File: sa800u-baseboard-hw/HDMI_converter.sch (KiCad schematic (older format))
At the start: 17 parts, among them U4 LT9611, Y2 ECS-1618-250-BN-TR

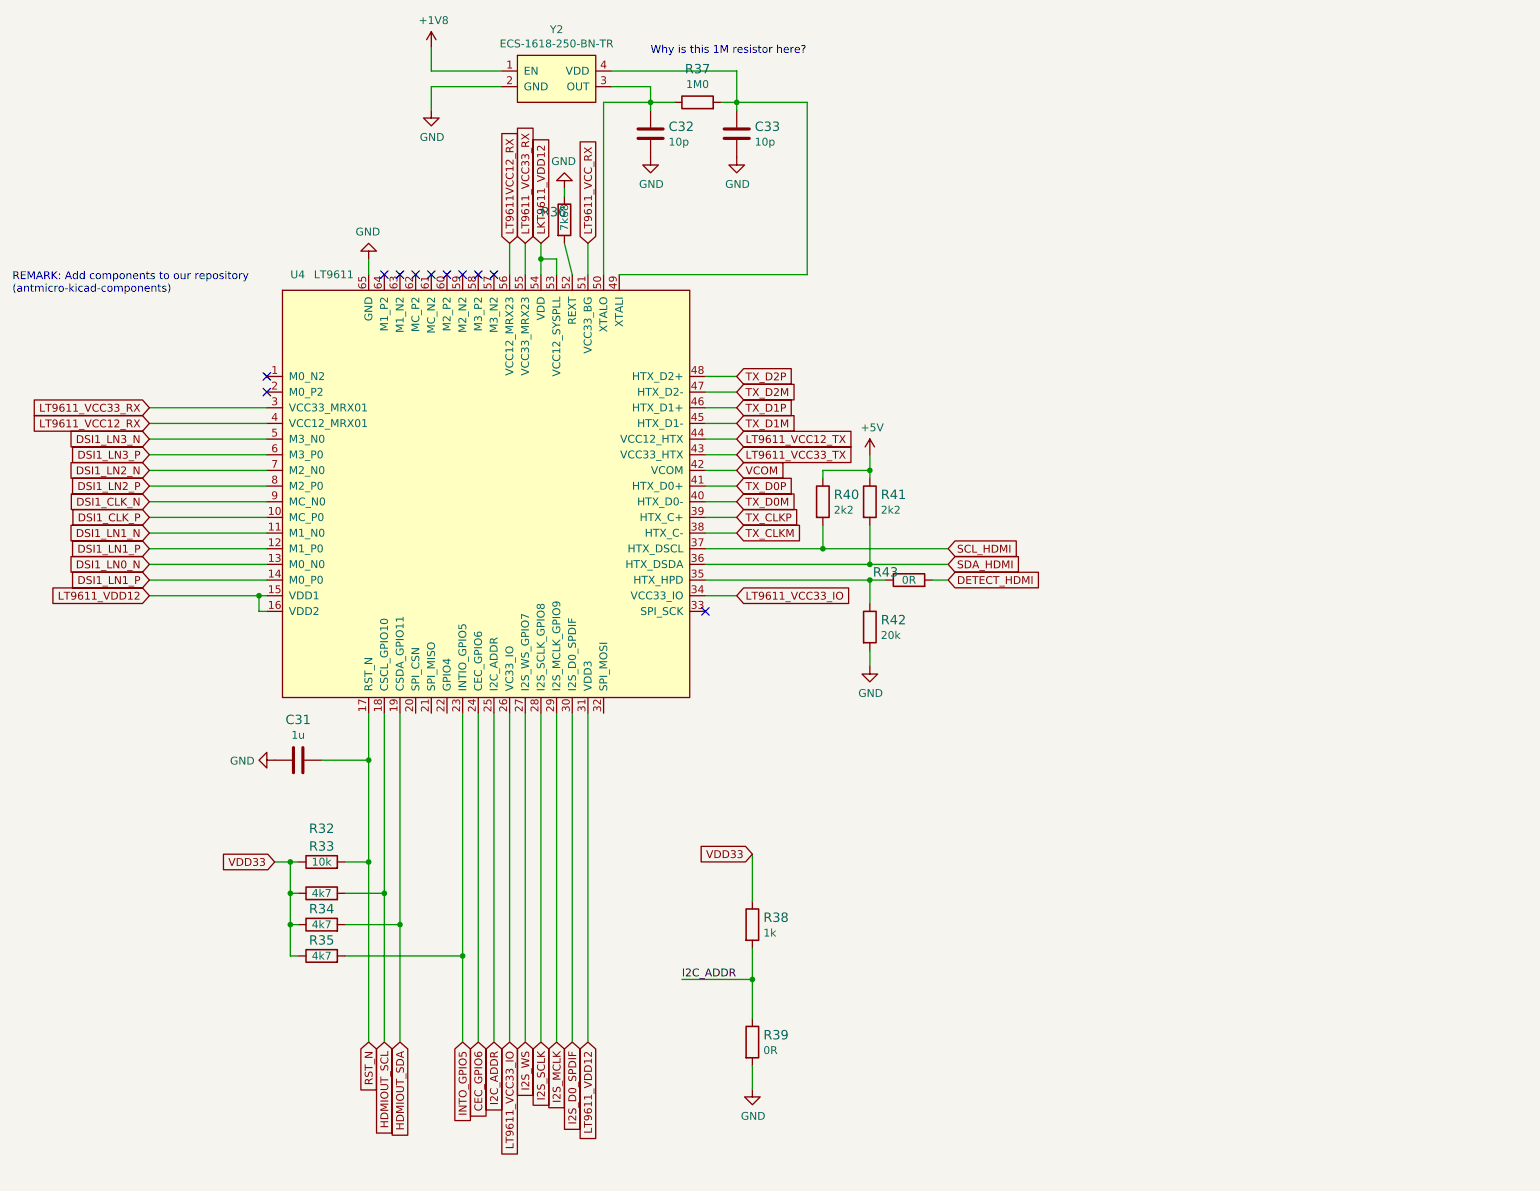
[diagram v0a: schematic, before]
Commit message: introducing minor genreal improvements
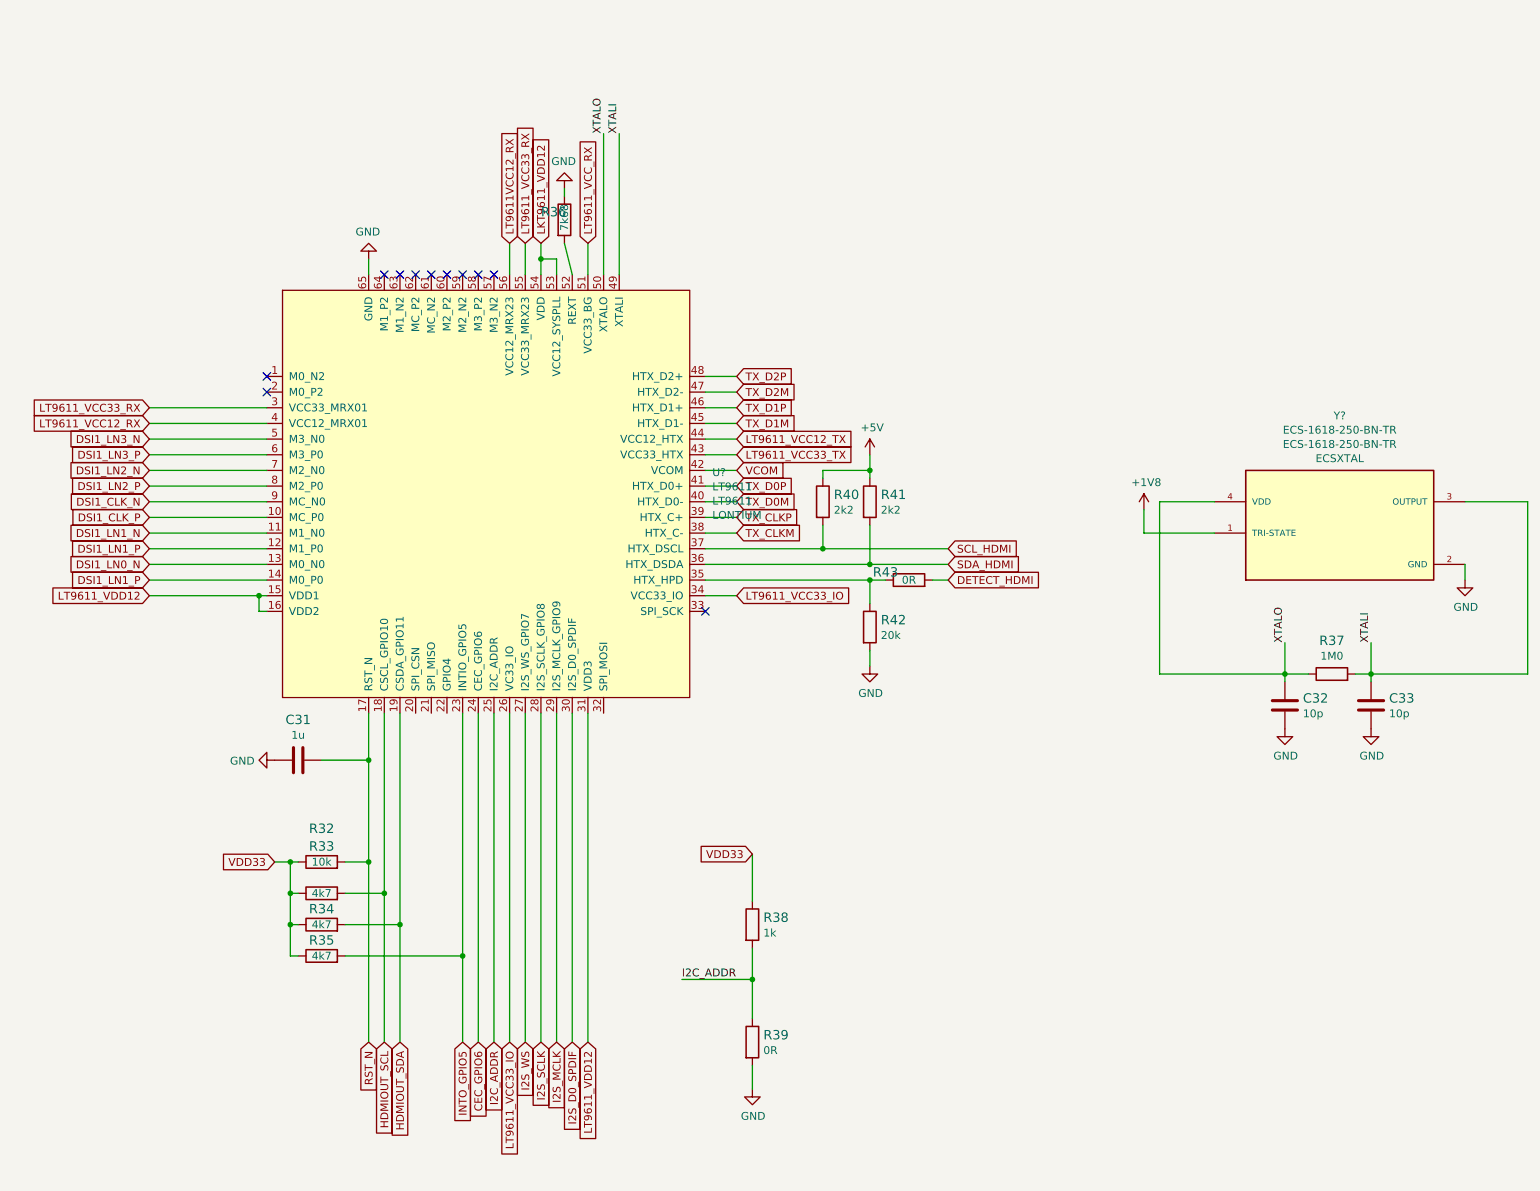
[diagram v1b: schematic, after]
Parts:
- removed U4: LT9611, symbol HDMI:LT9611
- removed Y2: ECS-1618-250-BN-TR, symbol Oscillators:ECS-1618-250-BN-TR
- added U?: LT9611, antmicro-footprints:LT9611, symbol antmicroInterfaceControllers:LT9611
- added Y?: ECS-1618-250-BN-TR, antmicro-footprints:OSC_ECS-1618-250-BN-TR, symbol antmicroOscillators:ECS-1618-250-BN-TR
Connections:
- net +1V8: now also Y?.1 (TRI-STATE)
- net CEC_GPIO6: now also U?.24 (CEC_GPIO6)
- net DSI1_CLK_N: now also U?.9 (MC_N0)
- net DSI1_CLK_P: now also U?.10 (MC_P0)
- net DSI1_LN0_N: now also U?.13 (M0_N0)
- net DSI1_LN1_N: now also U?.11 (M1_N0)
- net DSI1_LN1_P: now also U?.12 (M1_P0), U?.14 (M0_P0)
- net DSI1_LN2_N: now also U?.7 (M2_N0)
- net DSI1_LN2_P: now also U?.8 (M2_P0)
- net DSI1_LN3_N: now also U?.5 (M3_N0)
- net DSI1_LN3_P: now also U?.6 (M3_P0)
- net GND: now also U?.65 (GND), Y?.2 (GND)
- net HDMIOUT_SCL: now also U?.18 (CSCL_GPIO10)
- net HDMIOUT_SDA: now also U?.19 (CSDA_GPIO11)
- net I2C_ADDR: now also U?.25 (I2C_ADDR)
- net I2S_D0_SPDIF: now also U?.30 (I2S_D0_SPDIF)
- net I2S_MCLK: now also U?.29 (I2S_MCLK_GPIO9)
- net I2S_SCLK: now also U?.28 (I2S_SCLK_GPIO8)
- net I2S_WS: now also U?.27 (I2S_WS_GPIO7)
- net INTO_GPIO5: now also U?.23 (INTIO_GPIO5)
- net LKT9611_VDD12: now also U?.53 (VCC12_SYSPLL), U?.54 (VDD)
- net LT9611VCC12_RX: now also U?.56 (VCC12_MRX23)
- net LT9611_VCC12_RX: now also U?.4 (VCC12_MRX01)
- net LT9611_VCC12_TX: now also U?.44 (VCC12_HTX)
- net LT9611_VCC33_IO: now also U?.26 (VC33_IO), U?.34 (VCC33_IO)
- net LT9611_VCC33_RX: now also U?.3 (VCC33_MRX01), U?.55 (VCC33_MRX23)
- net LT9611_VCC33_TX: now also U?.43 (VCC33_HTX)
- net LT9611_VCC_RX: now also U?.51 (VCC33_BG)
- net LT9611_VDD12: now also U?.15 (VDD1), U?.16 (VDD2), U?.31 (VDD3)
- net RST_N: now also U?.17 (RST_N)
- net SCL_HDMI: now also U?.37 (HTX_DSCL)
- net SDA_HDMI: now also U?.36 (HTX_DSDA)
- net TX_CLKM: now also U?.38 (HTX_C-)
- net TX_CLKP: now also U?.39 (HTX_C+)
- net TX_D0M: now also U?.40 (HTX_D0-)
- net TX_D0P: now also U?.41 (HTX_D0+)
- net TX_D1M: now also U?.45 (HTX_D1-)
- net TX_D1P: now also U?.46 (HTX_D1+)
- net TX_D2M: now also U?.47 (HTX_D2-)
- net TX_D2P: now also U?.48 (HTX_D2+)
- net VCOM: now also U?.42 (VCOM)
- net at R42.1, R43.1: now also U?.35 (HTX_HPD)
- net XTALI: now reaches C33.1, R37.2
- net XTALI: now also U?.49 (XTALI), Y?.3 (OUTPUT)
- net XTALO: now reaches C32.1, R37.1
- net XTALO: now also U?.50 (XTALO), Y?.4 (VDD)
- net at R36.2: now also U?.52 (REXT)
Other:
- note removed: "REMARK: Add components to our repository \n(antmicro-kicad-components)"
- note removed: "Why is this 1M resistor here? \n"
- moved on the sheet: C32, C33, R37
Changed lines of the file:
@@
 Comment4 ""
 $EndDescr
-$Comp
-L HDMI:LT9611 U4
-U 1 1 61A0479A
-P 2250 2250
-F 0 "U4" H 2300 2350 50  0000 L CNN
-F 1 "LT9611" H 2450 2350 50  0000 L CNN
-F 2 "" H 1500 1950 50  0001 C CNN
-F 3 "" H 1500 1950 50  0001 C CNN
-	1    2250 2250
-	1    0    0    -1
-$EndComp
 Wire Wire Line
 	1400 3000 2150 3000
@@
 L power:GND #PWR?
 U 1 1 61A80E9F
-P 3200 1100
+P 9800 4100
 AR Path="/618E716E/61A80E9F" Ref="#PWR?"  Part="1"
 AR Path="/6197686D/61A80E9F" Ref="#PWR0115"  Part="1"
-F 0 "#PWR0115" H 3200 850 50  0001 C CNN
-F 1 "GND" H 3205 927 50  0000 C CNN
-F 2 "" H 3200 1100 50  0001 C CNN
-F 3 "" H 3200 1100 50  0001 C CNN
-	1    3200 1100
-	1    0    0    -1
-$EndComp
-Wire Wire Line
-	3200 950  3200 1100
-Wire Wire Line
-	3650 950  3200 950
+F 0 "#PWR0115" H 9800 3850 50  0001 C CNN
+F 1 "GND" H 9805 3927 50  0000 C CNN
+F 2 "" H 9800 4100 50  0001 C CNN
+F 3 "" H 9800 4100 50  0001 C CNN
+	1    9800 4100
+	1    0    0    -1
+$EndComp
 $Comp
 L power:+1V8 #PWR?
 U 1 1 61A80E97
-P 3200 700
+P 7750 3650
 AR Path="/618E716E/61A80E97" Ref="#PWR?"  Part="1"
 AR Path="/6197686D/61A80E97" Ref="#PWR0116"  Part="1"
-F 0 "#PWR0116" H 3200 550 50  0001 C CNN
-F 1 "+1V8" H 3215 873 50  0000 C CNN
-F 2 "" H 3200 700 50  0001 C CNN
-F 3 "" H 3200 700 50  0001 C CNN
-	1    3200 700
-	1    0    0    -1
-$EndComp
-Wire Wire Line
-	3200 850  3200 700
-Wire Wire Line
-	3650 850  3200 850
-$Comp
-L Oscillators:ECS-1618-250-BN-TR Y?
-U 1 1 61A80E8F
-P 3750 750
-AR Path="/618E716E/61A80E8F" Ref="Y?"  Part="1"
-AR Path="/6197686D/61A80E8F" Ref="Y2"  Part="1"
-F 0 "Y2" H 4000 915 50  0000 C CNN
-F 1 "ECS-1618-250-BN-TR" H 4000 824 50  0000 C CNN
-F 2 "" H 3950 800 50  0001 C CNN
-F 3 "" H 3950 800 50  0001 C CNN
-	1    3750 750
-	1    0    0    -1
-$EndComp
-Wire Wire Line
-	4350 950  4600 950
-Wire Wire Line
-	4600 950  4600 1050
-$Comp
-L antmicroCapacitors0402:C_10p_0402 C?
-U 1 1 61A80EAA
-P 4600 1250
-AR Path="/618E716E/61A80EAA" Ref="C?"  Part="1"
-AR Path="/6197686D/61A80EAA" Ref="C32"  Part="1"
-F 0 "C32" H 4715 1295 60  0000 L CNN
-F 1 "C_10p_0402" H 4600 1100 60  0001 C CNN
-F 2 "antmicro-footprints:0402-cap" H 4800 1450 60  0001 L CNN
-F 3 "" H 4600 1250 50  0001 C CNN
-F 4 "MULTICOMP" H 4800 1650 60  0001 L CNN "Manufacturer"
-F 5 "MC0402N100D500CT" H 4800 1550 60  0001 L CNN "MPN"
-F 6 "10p" H 4715 1197 50  0000 L CNN "Val"
-	1    4600 1250
-	1    0    0    -1
-$EndComp
-$Comp
-L power:GND #PWR?
-U 1 1 61A80EB0
-P 4600 1400
-AR Path="/618E716E/61A80EB0" Ref="#PWR?"  Part="1"
-AR Path="/6197686D/61A80EB0" Ref="#PWR0117"  Part="1"
-F 0 "#PWR0117" H 4600 1150 50  0001 C CNN
-F 1 "GND" H 4605 1227 50  0000 C CNN
-F 2 "" H 4600 1400 50  0001 C CNN
-F 3 "" H 4600 1400 50  0001 C CNN
-	1    4600 1400
-	1    0    0    -1
-$EndComp
-Wire Wire Line
-	4350 850  5150 850
-Wire Wire Line
-	5150 850  5150 1050
-$Comp
-L antmicroCapacitors0402:C_10p_0402 C?
-U 1 1 61A80EBB
-P 5150 1250
-AR Path="/618E716E/61A80EBB" Ref="C?"  Part="1"
-AR Path="/6197686D/61A80EBB" Ref="C33"  Part="1"
-F 0 "C33" H 5265 1295 60  0000 L CNN
-F 1 "C_10p_0402" H 5150 1100 60  0001 C CNN
-F 2 "antmicro-footprints:0402-cap" H 5350 1450 60  0001 L CNN
-F 3 "" H 5150 1250 50  0001 C CNN
-F 4 "MULTICOMP" H 5350 1650 60  0001 L CNN "Manufacturer"
-F 5 "MC0402N100D500CT" H 5350 1550 60  0001 L CNN "MPN"
-F 6 "10p" H 5265 1197 50  0000 L CNN "Val"
-	1    5150 1250
-	1    0    0    -1
-$EndComp
-$Comp
-L power:GND #PWR?
-U 1 1 61A80EC1
-P 5150 1400
-AR Path="/618E716E/61A80EC1" Ref="#PWR?"  Part="1"
-AR Path="/6197686D/61A80EC1" Ref="#PWR0118"  Part="1"
-F 0 "#PWR0118" H 5150 1150 50  0001 C CNN
-F 1 "GND" H 5155 1227 50  0000 C CNN
-F 2 "" H 5150 1400 50  0001 C CNN
-F 3 "" H 5150 1400 50  0001 C CNN
-	1    5150 1400
-	1    0    0    -1
-$EndComp
-Connection ~ 4600 1050
-Wire Wire Line
-	4600 1050 4600 1100
-$Comp
-L antmicroResistors0402:R_1M0_0402 R?
-U 1 1 61A80ECC
-P 4900 1050
-AR Path="/618E716E/61A80ECC" Ref="R?"  Part="1"
-AR Path="/6197686D/61A80ECC" Ref="R37"  Part="1"
-F 0 "R37" H 4900 1263 60  0000 C CNN
-F 1 "R_1M0_0402" H 4900 900 60  0001 C CNN
-F 2 "antmicro-footprints:0402-res" H 5100 1250 60  0001 L CNN
-F 3 "" H 4900 1050 50  0001 C CNN
-F 4 "TE CONNECTIVITY" H 5100 1450 60  0001 L CNN "Manufacturer"
-F 5 "CRG0402F1M0" H 5100 1350 60  0001 L CNN "MPN"
-F 6 "1M0" H 4900 1165 50  0000 C CNN "Val"
-	1    4900 1050
-	1    0    0    -1
-$EndComp
-Wire Wire Line
-	4600 1050 4750 1050
-Wire Wire Line
-	5050 1050 5150 1050
-Connection ~ 5150 1050
-Wire Wire Line
-	5150 1050 5150 1100
-Text Notes 4600 750  0    50   ~ 0
-Why is this 1M resistor here? \n
-Wire Wire Line
-	4600 1050 4300 1050
-Wire Wire Line
-	4300 1050 4300 2150
-Wire Wire Line
-	5150 1050 5600 1050
-Wire Wire Line
-	5600 1050 5600 2150
-Wire Wire Line
-	5600 2150 4400 2150
+F 0 "#PWR0116" H 7750 3500 50  0001 C CNN
+F 1 "+1V8" H 7765 3823 50  0000 C CNN
+F 2 "" H 7750 3650 50  0001 C CNN
+F 3 "" H 7750 3650 50  0001 C CNN
+	1    7750 3650
+	1    0    0    -1
+$EndComp
+Wire Wire Line
+	7750 3800 7750 3650
+Wire Wire Line
+	8200 3800 7750 3800
 Text GLabel 1400 3000 0    50   Input ~ 0
 LT9611_VCC33_RX
@@
 Text GLabel 4200 7050 3    50   Input ~ 0
 LT9611_VDD12
-Text Notes 525  2275 0    50   ~ 0
-REMARK: Add components to our repository \n(antmicro-kicad-components)
+$Comp
+L antmicroInterfaceControllers:LT9611 U?
+U 1 1 61A27AED
+P 2250 2250
+F 0 "U?" H 4994 1087 50  0000 L CNN
+F 1 "LT9611" H 4994 996 50  0000 L CNN
+F 2 "antmicro-footprints:LT9611" H 2250 2250 50  0001 C CNN
+F 3 "https://dev.antmicro.com/attachments/145681/LT9611_Datasheet_R2.0%20(1).pdf" H 2250 2250 50  0001 C CNN
+F 4 "LT9611" H 4994 905 50  0000 L CNN "MPN"
+F 5 "LONTIUM" H 4994 814 50  0000 L CNN "Manufacturer"
+	1    2250 2250
+	1    0    0    -1
+$EndComp
+$Comp
+L antmicroOscillators:ECS-1618-250-BN-TR Y?
+U 1 1 61A99388
+P 8400 3400
+F 0 "Y?" H 9000 3749 50  0000 C CNN
+F 1 "ECS-1618-250-BN-TR" H 9000 3658 50  0000 C CNN
+F 2 "antmicro-footprints:OSC_ECS-1618-250-BN-TR" H 8400 3400 50  0001 C CNN
+F 3 "https://ecsxtal.com/store/pdf/ECS_1618.pdf" H 8400 3400 50  0001 C CNN
+F 4 "ECS-1618-250-BN-TR" H 9000 3567 50  0000 C CNN "MPN"
+F 5 "ECSXTAL" H 9000 3476 50  0000 C CNN "Manufacturer"
+	1    8400 3400
+	1    0    0    -1
+$EndComp
+Wire Wire Line
+	9200 4700 9200 4750
+Connection ~ 9200 4700
+Wire Wire Line
+	9100 4700 9200 4700
+Wire Wire Line
+	8650 4700 8800 4700
+$Comp
+L antmicroResistors0402:R_1M0_0402 R?
+U 1 1 61A80ECC
+P 8950 4700
+AR Path="/618E716E/61A80ECC" Ref="R?"  Part="1"
+AR Path="/6197686D/61A80ECC" Ref="R37"  Part="1"
+F 0 "R37" H 8950 4913 60  0000 C CNN
+F 1 "R_1M0_0402" H 8950 4550 60  0001 C CNN
+F 2 "antmicro-footprints:0402-res" H 9150 4900 60  0001 L CNN
+F 3 "" H 8950 4700 50  0001 C CNN
+F 4 "TE CONNECTIVITY" H 9150 5100 60  0001 L CNN "Manufacturer"
+F 5 "CRG0402F1M0" H 9150 5000 60  0001 L CNN "MPN"
+F 6 "1M0" H 8950 4815 50  0000 C CNN "Val"
+	1    8950 4700
+	1    0    0    -1
+$EndComp
+Wire Wire Line
+	8650 4700 8650 4750
+Connection ~ 8650 4700
+$Comp
+L power:GND #PWR?
+U 1 1 61A80EC1
+P 9200 5050
+AR Path="/618E716E/61A80EC1" Ref="#PWR?"  Part="1"
+AR Path="/6197686D/61A80EC1" Ref="#PWR0118"  Part="1"
+F 0 "#PWR0118" H 9200 4800 50  0001 C CNN
+F 1 "GND" H 9205 4877 50  0000 C CNN
+F 2 "" H 9200 5050 50  0001 C CNN
+F 3 "" H 9200 5050 50  0001 C CNN
+	1    9200 5050
+	1    0    0    -1
+$EndComp
+$Comp
+L antmicroCapacitors0402:C_10p_0402 C?
+U 1 1 61A80EBB
+P 9200 4900
+AR Path="/618E716E/61A80EBB" Ref="C?"  Part="1"
+AR Path="/6197686D/61A80EBB" Ref="C33"  Part="1"
+F 0 "C33" H 9315 4945 60  0000 L CNN
+F 1 "C_10p_0402" H 9200 4750 60  0001 C CNN
+F 2 "antmicro-footprints:0402-cap" H 9400 5100 60  0001 L CNN
+F 3 "" H 9200 4900 50  0001 C CNN
+F 4 "MULTICOMP" H 9400 5300 60  0001 L CNN "Manufacturer"
+F 5 "MC0402N100D500CT" H 9400 5200 60  0001 L CNN "MPN"
+F 6 "10p" H 9315 4847 50  0000 L CNN "Val"
+	1    9200 4900
+	1    0    0    -1
+$EndComp
+Wire Wire Line
+	9200 4500 9200 4700
+$Comp
+L power:GND #PWR?
+U 1 1 61A80EB0
+P 8650 5050
+AR Path="/618E716E/61A80EB0" Ref="#PWR?"  Part="1"
+AR Path="/6197686D/61A80EB0" Ref="#PWR0117"  Part="1"
+F 0 "#PWR0117" H 8650 4800 50  0001 C CNN
+F 1 "GND" H 8655 4877 50  0000 C CNN
+F 2 "" H 8650 5050 50  0001 C CNN
+F 3 "" H 8650 5050 50  0001 C CNN
+	1    8650 5050
+	1    0    0    -1
+$EndComp
+$Comp
+L antmicroCapacitors0402:C_10p_0402 C?
+U 1 1 61A80EAA
+P 8650 4900
+AR Path="/618E716E/61A80EAA" Ref="C?"  Part="1"
+AR Path="/6197686D/61A80EAA" Ref="C32"  Part="1"
+F 0 "C32" H 8765 4945 60  0000 L CNN
+F 1 "C_10p_0402" H 8650 4750 60  0001 C CNN
+F 2 "antmicro-footprints:0402-cap" H 8850 5100 60  0001 L CNN
+F 3 "" H 8650 4900 50  0001 C CNN
+F 4 "MULTICOMP" H 8850 5300 60  0001 L CNN "Manufacturer"
+F 5 "MC0402N100D500CT" H 8850 5200 60  0001 L CNN "MPN"
+F 6 "10p" H 8765 4847 50  0000 L CNN "Val"
+	1    8650 4900
+	1    0    0    -1
+$EndComp
+Wire Wire Line
+	8200 3600 7850 3600
+Wire Wire Line
+	7850 3600 7850 4700
+Wire Wire Line
+	7850 4700 8650 4700
+Wire Wire Line
+	9800 3600 10200 3600
+Wire Wire Line
+	10200 3600 10200 4700
+Wire Wire Line
+	9200 4700 10200 4700
+Wire Wire Line
+	8650 4500 8650 4700
+Wire Wire Line
+	9800 4000 9800 4100
+Text Label 4300 1250 1    50   ~ 0
+XTALO
+Text Label 4400 1250 1    50   ~ 0
+XTALI
+Wire Wire Line
+	4300 1250 4300 2150
+Wire Wire Line
+	4400 1250 4400 2150
+Text Label 8650 4500 1    50   ~ 0
+XTALO
+Text Label 9200 4500 1    50   ~ 0
+XTALI
 $EndSCHEMATC
